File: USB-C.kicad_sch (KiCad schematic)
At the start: 35 parts, among them IC2 TPS2557QDRBTQ1, IC5 TPS2557QDRBTQ1, IC7 TPS2557QDRBTQ1, J10 USB_C_Receptacle, J5 USB_C_Receptacle_USB2.0_16P, J7 USB_C_Receptacle_USB2.0_16P

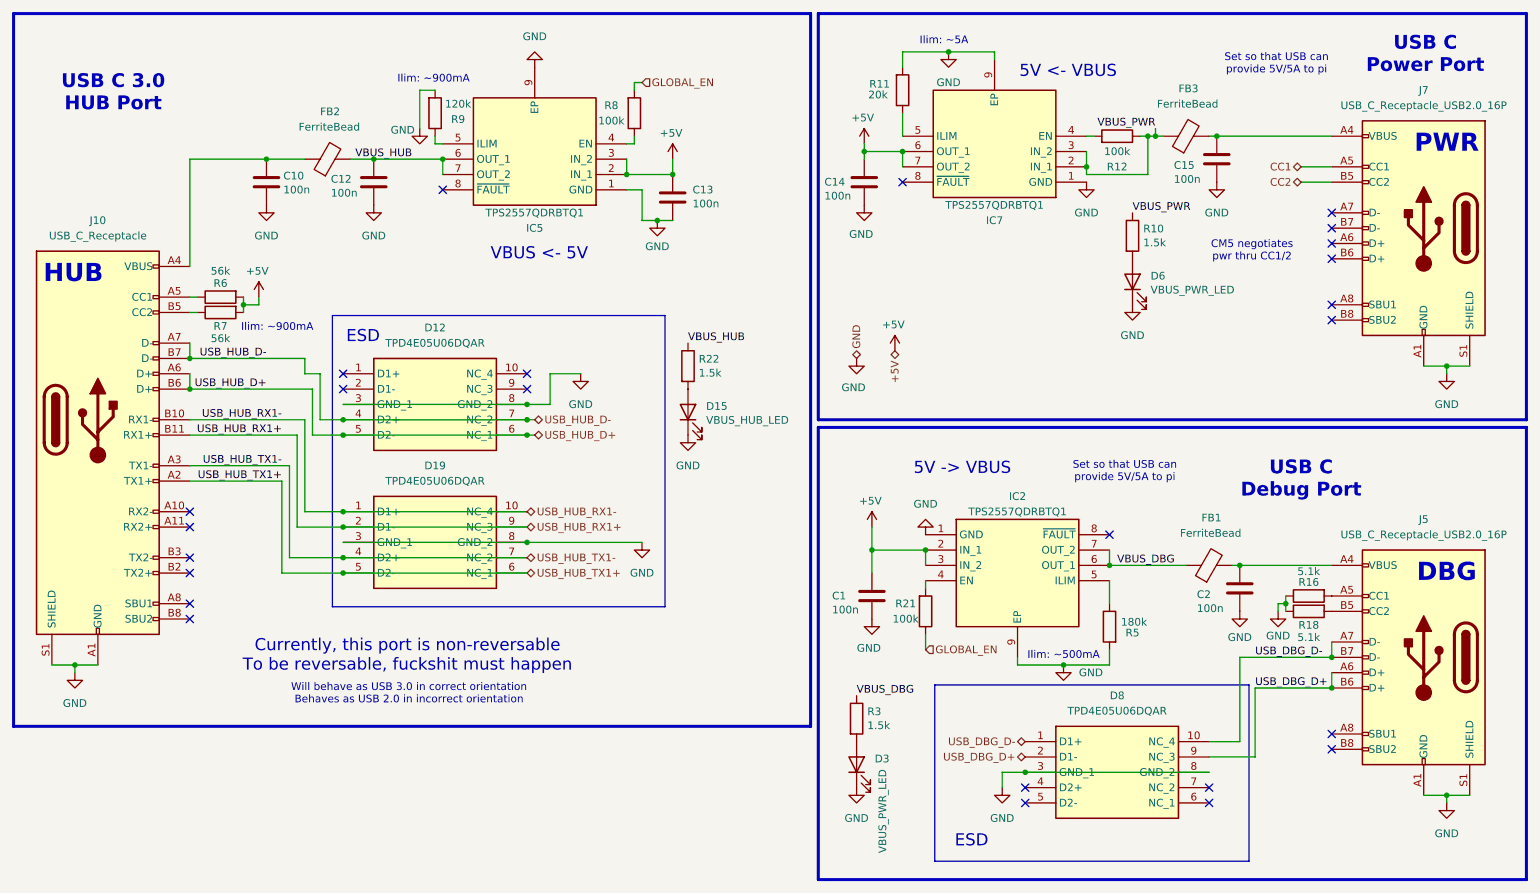
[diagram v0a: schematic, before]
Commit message: rrr
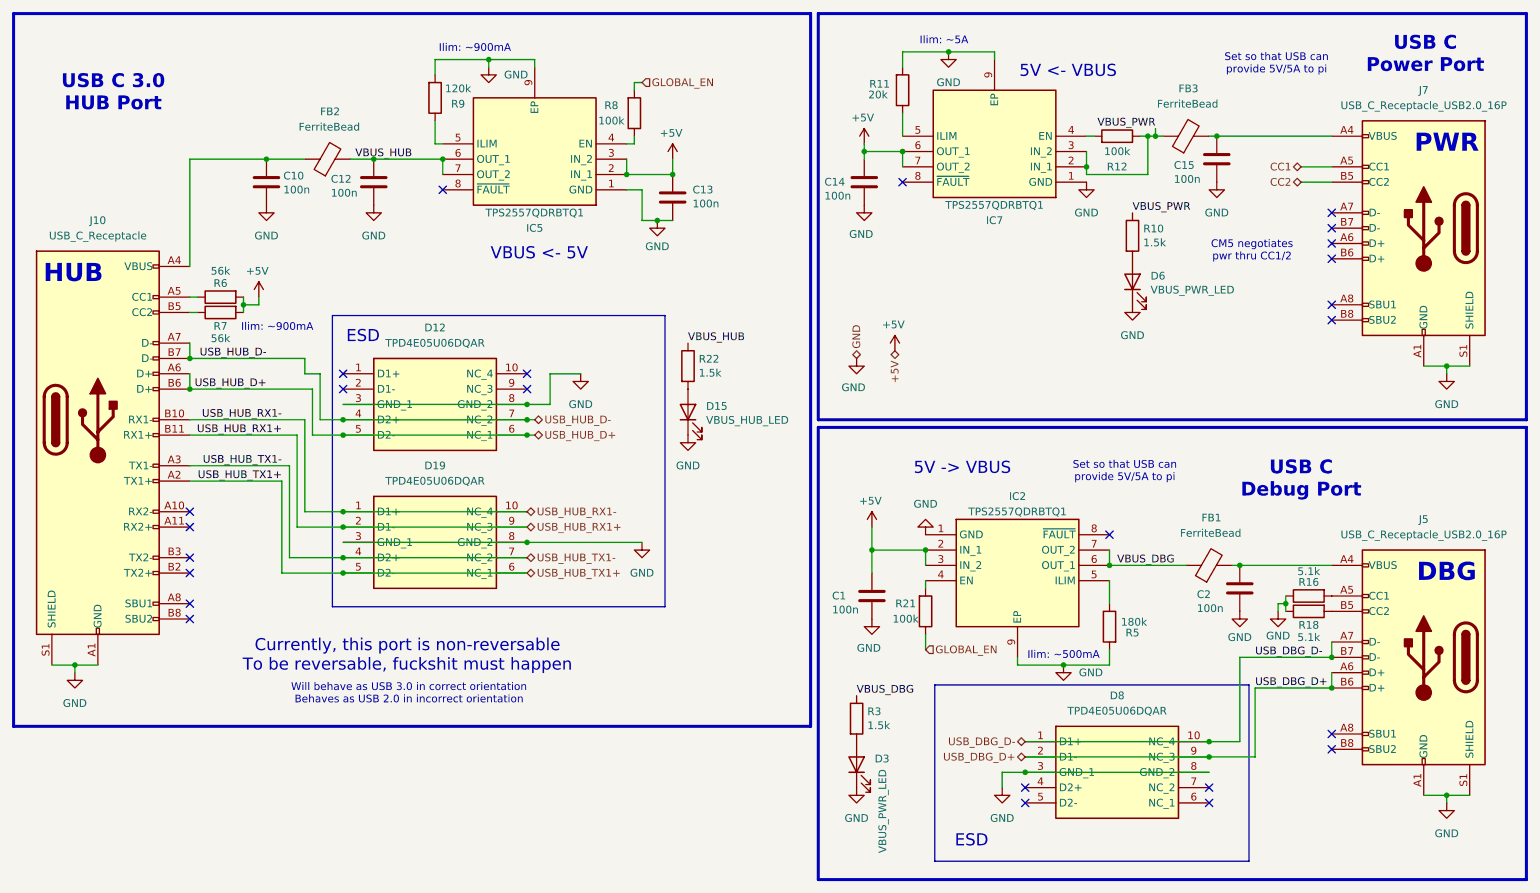
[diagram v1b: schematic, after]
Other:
- moved on the sheet: R9
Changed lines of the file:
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@@
 	(text "Ilim: ~900mA"
 		(exclude_from_sim no)
-		(at 92.456 26.162 0)
+		(at 99.314 21.082 0)
 		(effects
 			(font
@@
 	)
 	(junction
+		(at 220.98 135.89)
+		(diameter 0)
+		(color 0 0 0 0)
+	)
+	(junction
 		(at 204.47 106.68)
 		(diameter 0)
@@
 	)
 	(junction
+		(at 220.98 138.43)
+		(diameter 0)
+		(color 0 0 0 0)
+	)
+	(junction
 		(at 212.09 35.56)
 		(diameter 0)
@@
 	)
 	(junction
+		(at 101.6 22.86)
+		(diameter 0)
+		(color 0 0 0 0)
+	)
+	(junction
 		(at 226.06 106.68)
 		(diameter 0)
@@
 	(wire
 		(pts
-			(xy 92.71 36.83) (xy 92.71 35.56)
+			(xy 92.71 36.83) (xy 92.71 33.02)
 		)
 		(stroke
@@
 	(wire
 		(pts
+			(xy 109.22 22.86) (xy 109.22 24.13)
+		)
+		(stroke
+			(width 0)
+			(type default)
+		)
+	)
+	(wire
+		(pts
 			(xy 256.54 144.78) (xy 260.35 144.78)
 		)
@@
 	(wire
 		(pts
-			(xy 90.17 34.29) (xy 90.17 27.94)
-		)
-		(stroke
-			(width 0)
-			(type default)
-		)
-	)
-	(wire
-		(pts
 			(xy 69.85 100.33) (xy 77.47 100.33)
 		)
@@
 	(wire
 		(pts
-			(xy 90.17 27.94) (xy 92.71 27.94)
+			(xy 170.18 24.13) (xy 170.18 21.59)
 		)
 		(stroke
@@
 	(wire
 		(pts
-			(xy 170.18 24.13) (xy 170.18 21.59)
+			(xy 204.47 120.65) (xy 204.47 123.19)
 		)
 		(stroke
@@
 	(wire
 		(pts
-			(xy 204.47 120.65) (xy 204.47 123.19)
+			(xy 256.54 73.66) (xy 260.35 73.66)
 		)
 		(stroke
@@
 	(wire
 		(pts
-			(xy 256.54 73.66) (xy 260.35 73.66)
+			(xy 212.09 34.29) (xy 212.09 35.56)
 		)
 		(stroke
@@
 	(wire
 		(pts
-			(xy 212.09 34.29) (xy 212.09 35.56)
+			(xy 92.71 25.4) (xy 92.71 22.86)
 		)
 		(stroke
@@
 	(wire
 		(pts
+			(xy 92.71 22.86) (xy 101.6 22.86)
+		)
+		(stroke
+			(width 0)
+			(type default)
+		)
+	)
+	(wire
+		(pts
 			(xy 222.25 35.56) (xy 241.3 35.56)
 		)
@@
 	(wire
 		(pts
+			(xy 190.5 138.43) (xy 220.98 138.43)
+		)
+		(stroke
+			(width 0)
+			(type default)
+		)
+	)
+	(wire
+		(pts
+			(xy 190.5 135.89) (xy 220.98 135.89)
+		)
+		(stroke
+			(width 0)
+			(type default)
+		)
+	)
+	(wire
+		(pts
 			(xy 67.31 92.71) (xy 52.07 92.71)
 		)
@@
 	(wire
 		(pts
+			(xy 101.6 22.86) (xy 109.22 22.86)
+		)
+		(stroke
+			(width 0)
+			(type default)
+		)
+	)
+	(wire
+		(pts
 			(xy 210.82 35.56) (xy 212.09 35.56)
 		)
@@
 	(wire
 		(pts
+			(xy 101.6 24.13) (xy 101.6 22.86)
+		)
+		(stroke
+			(width 0)
+			(type default)
+		)
+	)
+	(wire
+		(pts
 			(xy 71.12 74.93) (xy 73.66 74.93)
 		)
@@
 	(symbol
 		(lib_id "Device:R")
-		(at 92.71 31.75 0)
+		(at 92.71 29.21 0)
 		(mirror x)
 		(unit 1)
@@
 		(dnp no)
 		(property "Reference" "R9"
-			(at 96.52 32.766 0)
+			(at 96.52 30.226 0)
 			(effects
 				(font
@@
 		)
 		(property "Value" "120k"
-			(at 96.52 30.226 0)
+			(at 96.52 27.686 0)
 			(effects
 				(font
@@
 		)
 		(property "Footprint" "Resistor_SMD:R_0603_1608Metric_Pad0.98x0.95mm_HandSolder"
-			(at 90.932 31.75 90)
+			(at 90.932 29.21 90)
 			(effects
 				(font
@@
 		)
 		(property "Datasheet" "~"
-			(at 92.71 31.75 0)
+			(at 92.71 29.21 0)
 			(effects
 				(font
@@
 		)
 		(property "Description" "Resistor"
-			(at 92.71 31.75 0)
+			(at 92.71 29.21 0)
 			(effects
 				(font
@@
 		)
 		(property "P/N" ""
-			(at 92.71 31.75 0)
+			(at 92.71 29.21 0)
 			(effects
 				(font
@@
 	(symbol
 		(lib_id "power:GND")
-		(at 109.22 24.13 180)
+		(at 101.6 24.13 0)
 		(unit 1)
 		(exclude_from_sim no)
@@
 		(fields_autoplaced yes)
 		(property "Reference" "#PWR074"
-			(at 109.22 17.78 0)
+			(at 101.6 30.48 0)
 			(effects
 				(font
@@
 		)
 		(property "Value" "GND"
-			(at 109.22 19.05 0)
+			(at 104.14 25.3999 0)
 			(effects
 				(font
 					(size 1.27 1.27)
 				)
+				(justify left)
 			)
 		)
 		(property "Footprint" ""
-			(at 109.22 24.13 0)
+			(at 101.6 24.13 0)
 			(effects
 				(font
@@
 		)
 		(property "Datasheet" ""
-			(at 109.22 24.13 0)
+			(at 101.6 24.13 0)
 			(effects
 				(font
@@
 		)
 		(property "Description" "Power symbol creates a global label with name \"GND\" , ground"
-			(at 109.22 24.13 0)
+			(at 101.6 24.13 0)
 			(effects
 				(font
@@
 					(unit 1)
 				)
-			)
-		)
-	)
-	(symbol
-		(lib_id "power:GND")
-		(at 90.17 34.29 0)
-		(unit 1)
-		(exclude_from_sim no)
-		(in_bom yes)
-		(on_board yes)
-		(dnp no)
-		(property "Reference" "#PWR093"
-			(at 90.17 40.64 0)
-			(effects
-				(font
-					(size 1.27 1.27)
-				)
-				(hide yes)
-			)
-		)
-		(property "Value" "GND"
-			(at 85.344 34.544 0)
-			(effects
-				(font
-					(size 1.27 1.27)
-				)
-				(justify left)
-			)
-		)
-		(property "Footprint" ""
-			(at 90.17 34.29 0)
-			(effects
-				(font
-					(size 1.27 1.27)
-				)
-				(hide yes)
-			)
-		)
-		(property "Datasheet" ""
-			(at 90.17 34.29 0)
-			(effects
-				(font
-					(size 1.27 1.27)
-				)
-				(hide yes)
-			)
-		)
-		(property "Description" "Power symbol creates a global label with name \"GND\" , ground"
-			(at 90.17 34.29 0)
-			(effects
-				(font
-					(size 1.27 1.27)
-				)
-				(hide yes)
-			)
-		)
-		(pin "1"
-		)
-		(instances
-			(project "PiBoard"
-				(path "/e4d65698-b8ec-4bf6-9f2b-a5010377155a/2dec5fd6-8756-425d-9ae9-2f1c2fc4e6c1/65247ae0-83ec-4f51-af4d-84b2c055b0d6"
-					(reference "#PWR093")
-					(unit 1)
-				)

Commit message: frank
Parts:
- J10: Data (none) -> https://www.molex.com/en-us/products/part-detail/2216080001; P/N 105450-0101 -> 221608-0001
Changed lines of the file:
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@@
 			)
 		)
-		(property "P/N" "105450-0101"
+		(property "P/N" "221608-0001"
 			(at 36.83 82.55 0)
 			(effects
+				(font
+					(size 1.27 1.27)
+				)
+				(hide yes)
+			)
+		)
+		(property "Data" "https://www.molex.com/en-us/products/part-detail/2216080001"
+			(at 36.83 82.55 0)
+			(effects
